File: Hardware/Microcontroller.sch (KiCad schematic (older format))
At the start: 22 parts

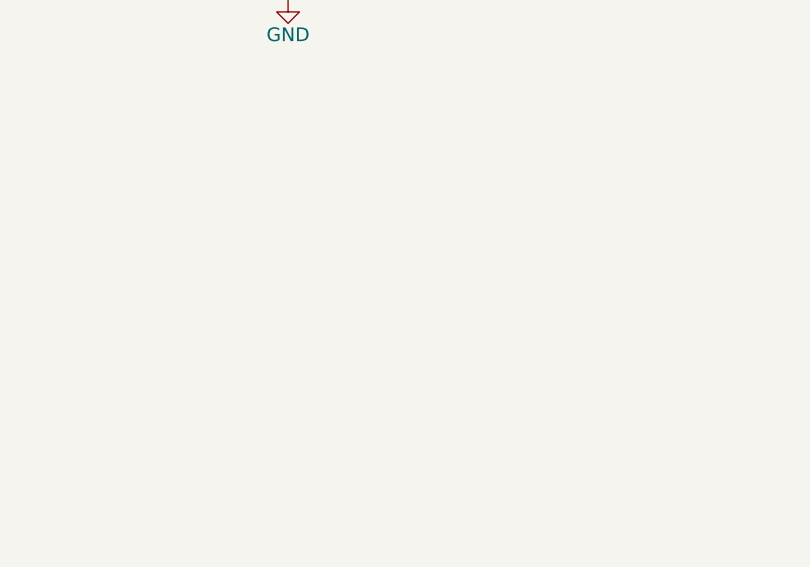
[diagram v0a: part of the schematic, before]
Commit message: Update general layout
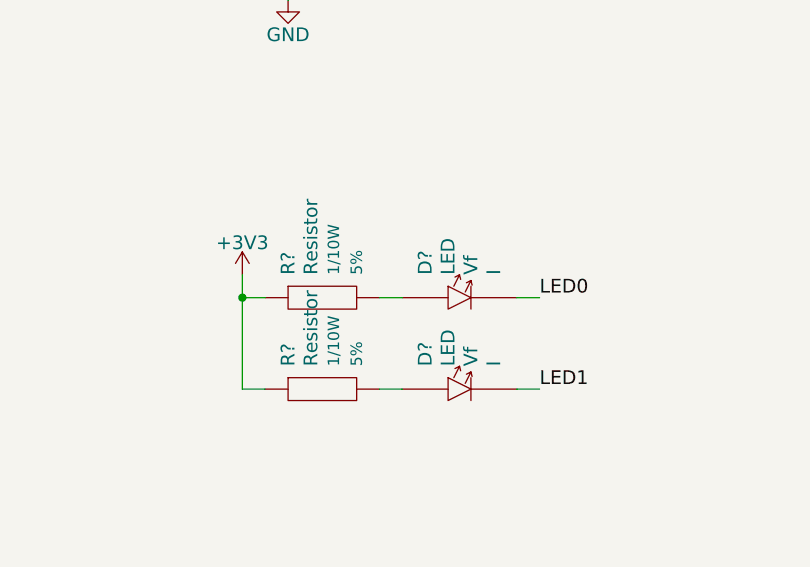
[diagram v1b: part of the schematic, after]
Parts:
- added D? (x2): LED, symbol LED
- added R? (x2): Resistor, symbol Resistor
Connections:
- net +3V3: now also R?.1, R?.1
- new net: D?.A, R?.2 (x2)
- new net LED0: D?.C
- new net LED1: D?.C
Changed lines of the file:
@@
 Text Notes 9100 1500 0    60   ~ 0
 DAC2
+$Comp
+L LED D?
+U 1 1 54A1A4D6
+P 5150 3300
+F 0 "D?" V 5000 3400 60  0000 L CNN
+F 1 "LED" V 5100 3400 60  0000 L CNN
+F 2 "" H 5150 3300 60  0000 C CNN
+F 3 "" H 5150 3300 60  0000 C CNN
+F 4 "Value" H 5150 3300 60  0001 C CNN "Manufacturer"
+F 5 "Value" H 5150 3300 60  0001 C CNN "Manufacturer Part #"
+F 6 "Value" H 5150 3300 60  0001 C CNN "Vendor"
+F 7 "Value" H 5150 3300 60  0001 C CNN "Vendor Part #"
+F 8 "Vf" V 5200 3400 60  0000 L CNN "Forward Voltage"
+F 9 "I" V 5300 3400 60  0000 L CNN "Current"
+	1    5150 3300
+	1    0    0    -1
+$EndComp
+$Comp
+L LED D?
+U 1 1 54A1A544
+P 5150 3700
+F 0 "D?" V 5000 3800 60  0000 L CNN
+F 1 "LED" V 5100 3800 60  0000 L CNN
+F 2 "" H 5150 3700 60  0000 C CNN
+F 3 "" H 5150 3700 60  0000 C CNN
+F 4 "Value" H 5150 3700 60  0001 C CNN "Manufacturer"
+F 5 "Value" H 5150 3700 60  0001 C CNN "Manufacturer Part #"
+F 6 "Value" H 5150 3700 60  0001 C CNN "Vendor"
+F 7 "Value" H 5150 3700 60  0001 C CNN "Vendor Part #"
+F 8 "Vf" V 5200 3800 60  0000 L CNN "Forward Voltage"
+F 9 "I" V 5300 3800 60  0000 L CNN "Current"
+	1    5150 3700
+	1    0    0    -1
+$EndComp
+$Comp
+L Resistor R?
+U 1 1 54A1A58D
+P 4550 3300
+F 0 "R?" V 4400 3400 60  0000 L CNN
+F 1 "Resistor" V 4500 3400 60  0000 L CNN
+F 2 "" H 4450 3300 60  0001 C CNN
+F 3 "" H 4550 3400 60  0001 C CNN
+F 4 "Value" H 4550 3300 60  0001 C CNN "Manufacturer"
+F 5 "Value" H 4550 3300 60  0001 C CNN "Manufacturer Part #"
+F 6 "Value" H 4550 3300 60  0001 C CNN "Vendor"
+F 7 "Value" H 4550 3300 60  0001 C CNN "Vendor Part #"
+F 8 "1/10W" V 4600 3400 50  0000 L CNN "Power"
+F 9 "5%" V 4700 3400 50  0000 L CNN "Tolerance"
+	1    4550 3300
+	1    0    0    -1
+$EndComp
+$Comp
+L Resistor R?
+U 1 1 54A1A5F4
+P 4550 3700
+F 0 "R?" V 4400 3800 60  0000 L CNN
+F 1 "Resistor" V 4500 3800 60  0000 L CNN
+F 2 "" H 4450 3700 60  0001 C CNN
+F 3 "" H 4550 3800 60  0001 C CNN
+F 4 "Value" H 4550 3700 60  0001 C CNN "Manufacturer"
+F 5 "Value" H 4550 3700 60  0001 C CNN "Manufacturer Part #"
+F 6 "Value" H 4550 3700 60  0001 C CNN "Vendor"
+F 7 "Value" H 4550 3700 60  0001 C CNN "Vendor Part #"
+F 8 "1/10W" V 4600 3800 50  0000 L CNN "Power"
+F 9 "5%" V 4700 3800 50  0000 L CNN "Tolerance"
+	1    4550 3700
+	1    0    0    -1
+$EndComp
+$Comp
+L +3V3 #PWR?
+U 1 1 54A1A643
+P 4200 3200
+F 0 "#PWR?" H 4200 3050 60  0001 C CNN
+F 1 "+3V3" H 4200 3340 60  0000 C CNN
+F 2 "" H 4200 3200 60  0000 C CNN
+F 3 "" H 4200 3200 60  0000 C CNN
+	1    4200 3200
+	1    0    0    -1
+$EndComp
+Wire Wire Line
+	4200 3200 4200 3700
+Wire Wire Line
+	4200 3700 4300 3700
+Wire Wire Line
+	4300 3300 4200 3300
+Connection ~ 4200 3300
+Text Label 5500 3300 0    60   ~ 0
+LED0
+Text Label 5500 3700 0    60   ~ 0
+LED1
+Wire Wire Line
+	4800 3300 4900 3300
+Wire Wire Line
+	4800 3700 4900 3700
+Wire Wire Line
+	5400 3300 5500 3300
+Wire Wire Line
+	5400 3700 5500 3700
 $EndSCHEMATC
